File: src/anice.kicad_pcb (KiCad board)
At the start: 4 copper layers, 65.6 x 34 mm, 100 parts, among them J1 Conn_02x20_Counter_Clockwise, J2 Micro_SD_Card_Det1, J3 USB_C_Receptacle_USB2.0_14P, J4 USB_C_Receptacle_USB2.0_14P, J5 USB_C_Receptacle_USB2.0_14P, J7 HDMI_C_1.3, U1 ECP5U_12_CABGA256, U10 W9825G6KH-6, U11 W25Q128JVS, U12 TLV62569DRL, U13 TLV62569DRL, U14 TLV62569DRL, U5 TPD2EUSB30, U6 TPD2EUSB30, U7 FT231XQ, U8 TPD2EUSB30, U9 PCA9306DC1, Y1 ECS-2520MV-xxx-xx

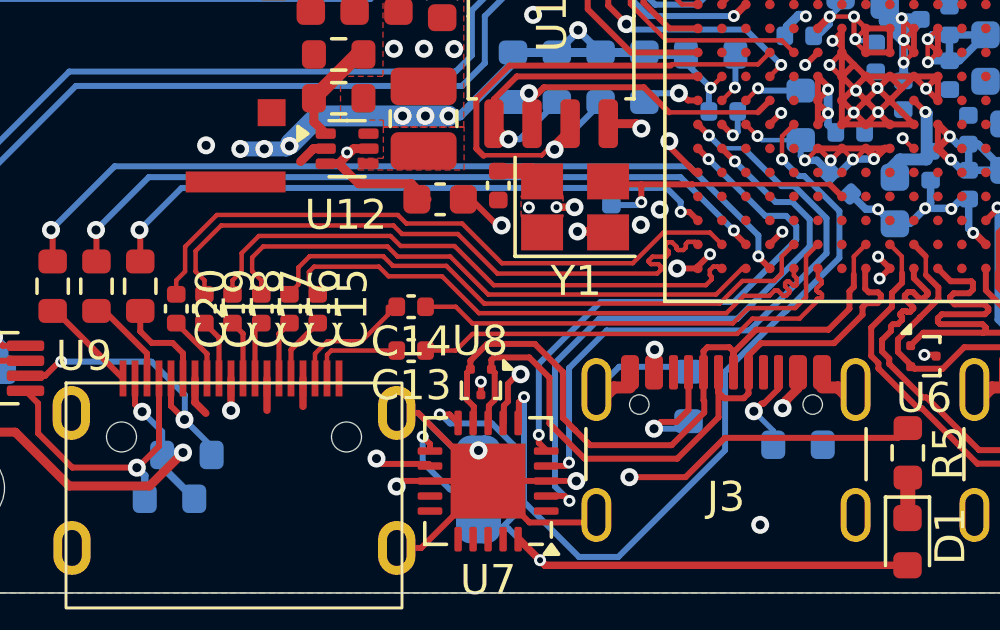
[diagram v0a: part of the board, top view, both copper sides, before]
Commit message: Tidy project
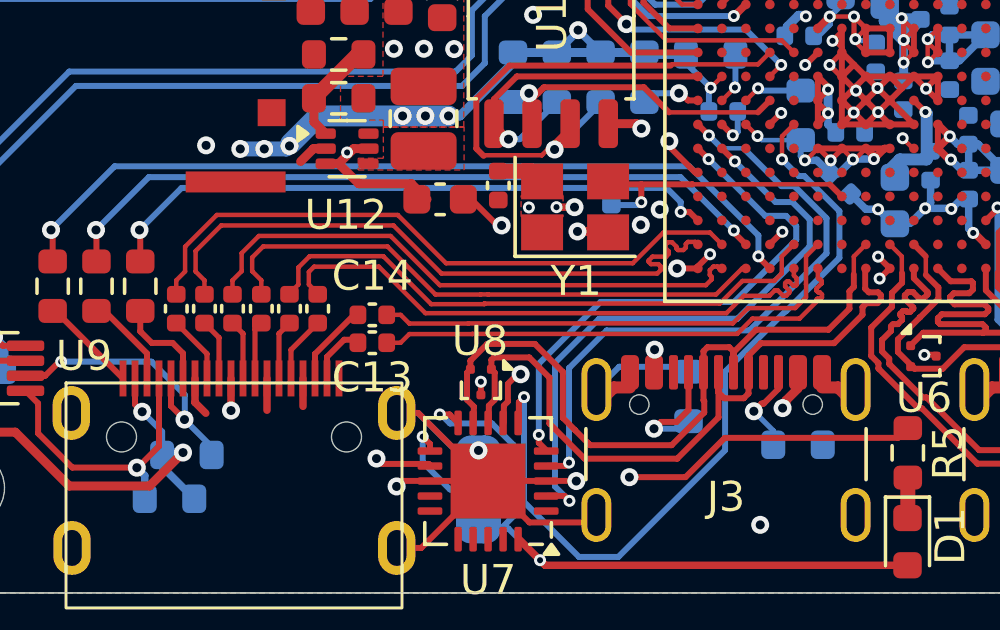
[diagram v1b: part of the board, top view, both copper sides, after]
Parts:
- moved C14 1.32 mm to (119.0, 95.7)
- moved C13 1.32 mm to (119.0, 96.7)
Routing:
- net FPDI_D2+: track 14.9 -> 16.4 mm
- net FPDI_D2-: track 14.9 -> 16.4 mm
- net Net-(J7-D2-): track 4.06 -> 2.85 mm
- net Net-(J7-D2+): track 2.88 -> 2.01 mm
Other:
- board text added: "Change files on the right side!!! -> These two pcbs will be joined together physically Scroll to zoom, Right click & drag to pan"
- board text removed: "Change files on the right side!!! -> These two pcbs will be joined together physically"
